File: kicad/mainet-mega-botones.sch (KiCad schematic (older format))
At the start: 6 parts, among them SW1 SW_Push_LED, SW2 SW_Push_LED, SW3 SW_Push_LED, SW4 SW_Push_LED, SW6 SW_Push_LED, SW7 SW_Push_LED

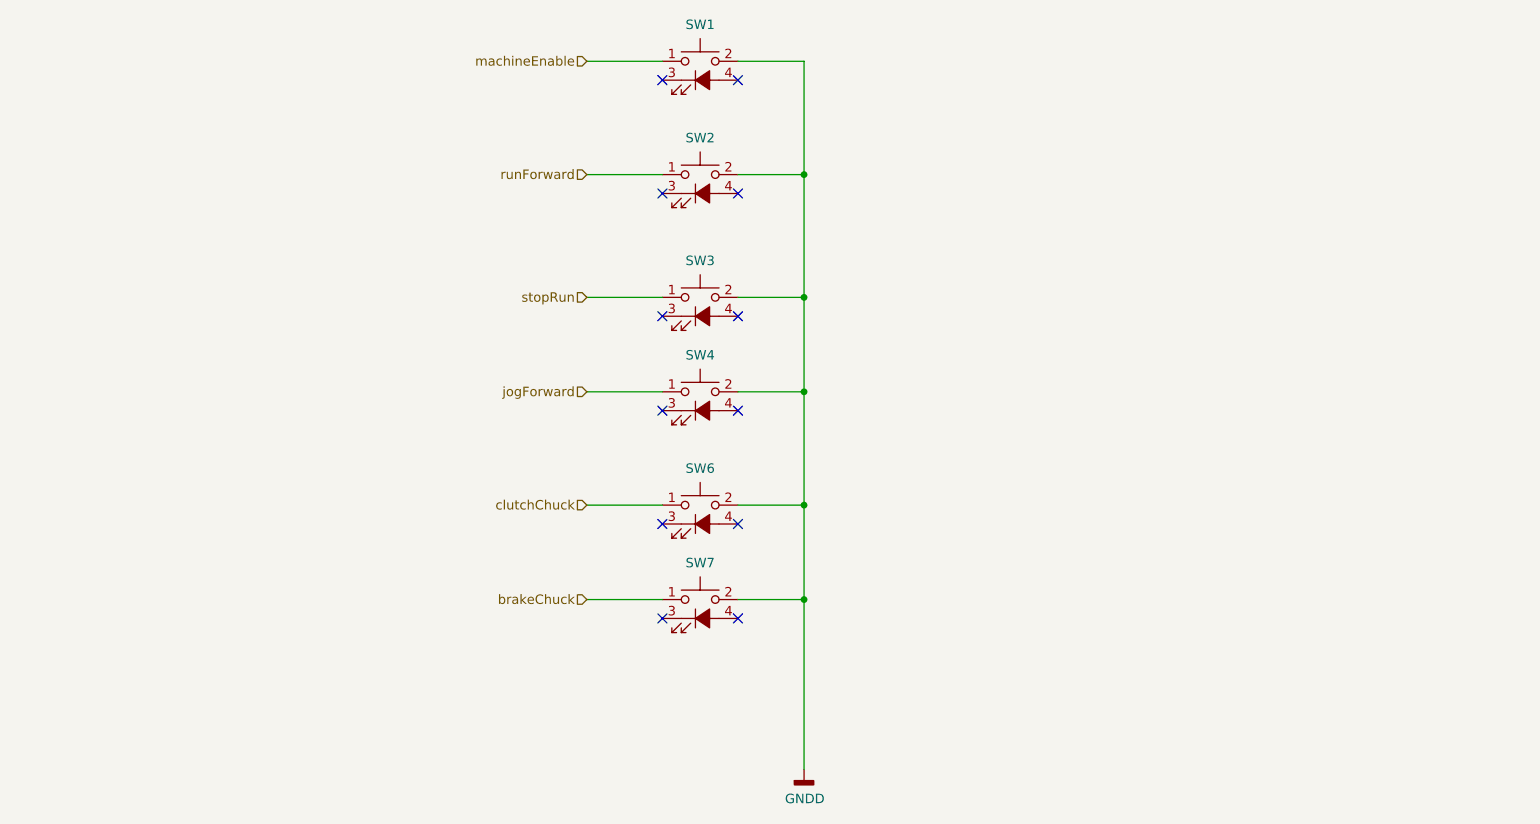
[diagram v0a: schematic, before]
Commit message: KICAD: Actualizar .sch para agregar cambio de giro
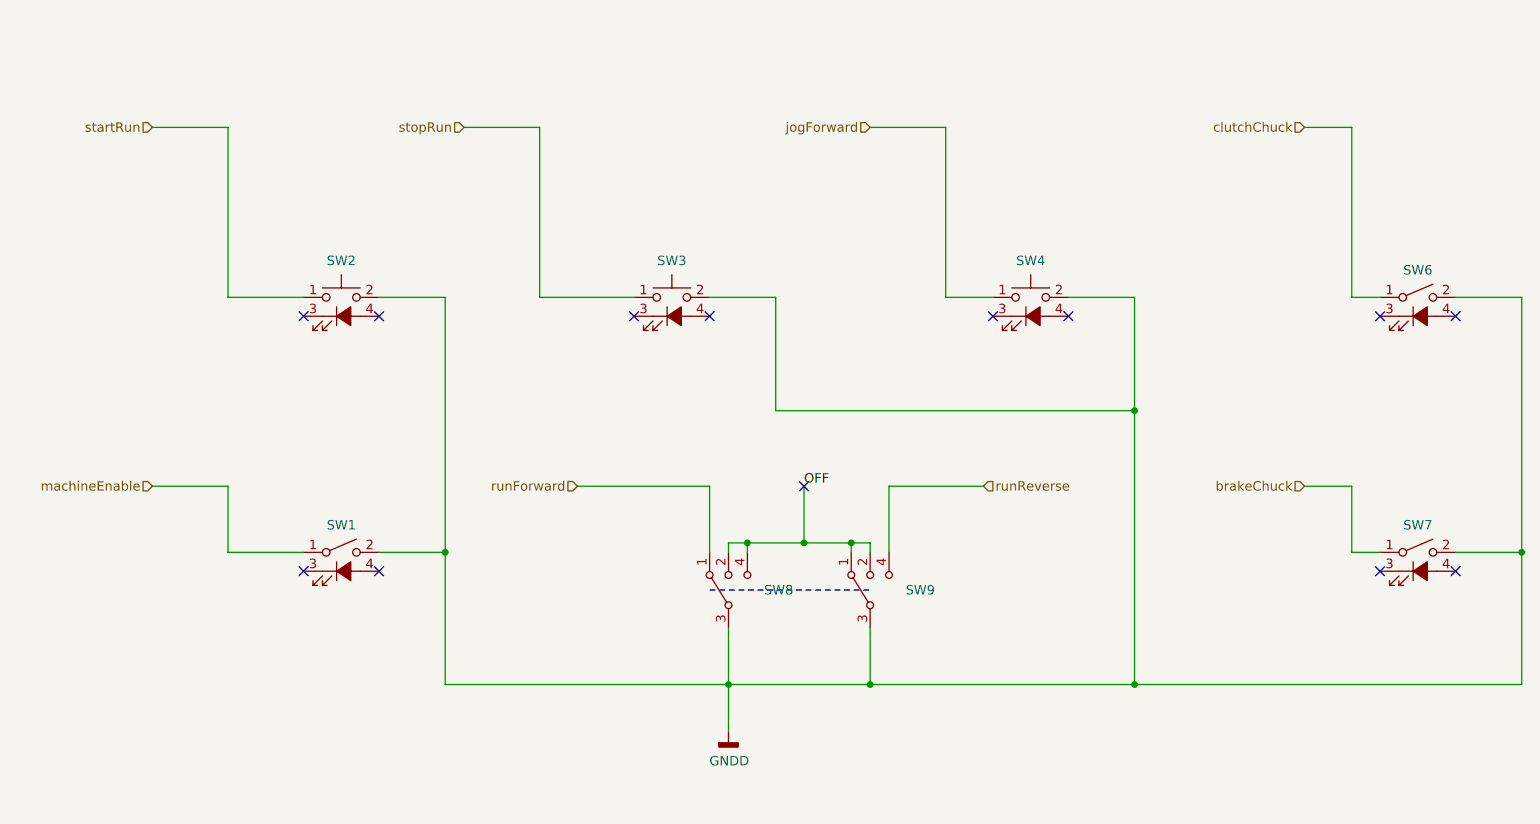
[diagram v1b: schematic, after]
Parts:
- removed SW1, SW6, SW7: SW_Push_LED, symbol Switch:SW_Push_LED
- added SW1, SW6, SW7: SW_SPST_LED, symbol Switch:SW_SPST_LED
- added SW8, SW9: SW_SP3T, symbol Switch:SW_SP3T
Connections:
- net GNDD: now also SW1.2, SW6.2, SW7.2, SW8.3, SW9.3
- net brakeChuck: now also SW7.1
- net clutchChuck: now also SW6.1
- net machineEnable: now also SW1.1
- net runForward: now also SW8.1; no longer SW2.1
- new net OFF: SW8.2, SW8.4, SW9.1, SW9.2
- new net runReverse: SW9.4
- new net startRun: SW2.1
- no-connect marks 12 -> 13
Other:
- moved on the sheet: SW2, SW3, SW4
